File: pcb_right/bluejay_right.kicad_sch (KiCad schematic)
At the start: 60 parts, among them J2 SJ-43514, U2 MCP23017

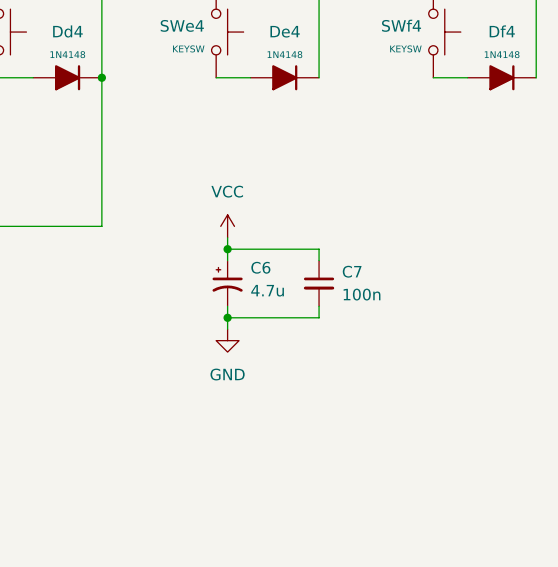
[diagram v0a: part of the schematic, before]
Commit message: Routing of right PCB
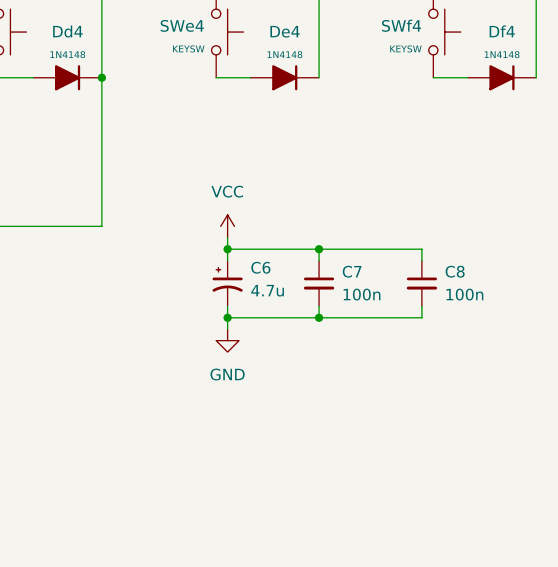
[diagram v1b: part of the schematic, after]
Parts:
- added C8: 100n, BlueJay footprints:C_Disc_D4.3mm_W1.9mm_P5.00mm, symbol BlueJaySymbolLibrary:C_Small
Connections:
- net GND: now also C8.2
- net VCC: now also C8.1
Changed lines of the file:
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@@
   (junction (at 146.05 62.23) (diameter 0) (color 0 0 0 0)
   )
+  (junction (at 229.87 111.76) (diameter 0) (color 0 0 0 0)
+  )
   (junction (at 219.71 111.76) (diameter 0) (color 0 0 0 0)
   )
@@
   )
   (junction (at 205.74 72.39) (diameter 0) (color 0 0 0 0)
+  )
+  (junction (at 229.87 104.14) (diameter 0) (color 0 0 0 0)
   )
   (junction (at 152.4 101.6) (diameter 0) (color 0 0 0 0)
@@
     (stroke (width 0) (type default) (color 0 0 0 0))
   )
+  (wire (pts (xy 241.3 111.76) (xy 241.3 110.49))
+    (stroke (width 0) (type default) (color 0 0 0 0))
+  )
   (wire (pts (xy 152.4 90.17) (xy 152.4 101.6))
     (stroke (width 0) (type default) (color 0 0 0 0))
@@
     (stroke (width 0) (type default) (color 0 0 0 0))
   )
+  (wire (pts (xy 229.87 111.76) (xy 241.3 111.76))
+    (stroke (width 0) (type default) (color 0 0 0 0))
+  )
   (wire (pts (xy 21.59 91.44) (xy 27.94 91.44))
     (stroke (width 0) (type default) (color 0 0 0 0))
@@
     (stroke (width 0) (type default) (color 0 0 0 0))
   )
+  (wire (pts (xy 229.87 104.14) (xy 241.3 104.14))
+    (stroke (width 0) (type default) (color 0 0 0 0))
+  )
   (wire (pts (xy 222.25 72.39) (xy 218.44 72.39))
     (stroke (width 0) (type default) (color 0 0 0 0))
@@
   )
   (wire (pts (xy 92.71 91.44) (xy 85.09 91.44))
+    (stroke (width 0) (type default) (color 0 0 0 0))
+  )
+  (wire (pts (xy 241.3 104.14) (xy 241.3 105.41))
     (stroke (width 0) (type default) (color 0 0 0 0))
   )
@@
     (pin "1")
   )
+  (symbol (lib_id "BlueJaySymbolLibrary:C_Small") (at 241.3 107.95 0) (unit 1)
+    (in_bom yes) (on_board yes) (fields_autoplaced)
+    (property "Reference" "C8" (id 0) (at 243.84 106.6862 0)
+      (effects (font (size 1.27 1.27)) (justify left))
+    )
+    (property "Value" "100n" (id 1) (at 243.84 109.2262 0)
+      (effects (font (size 1.27 1.27)) (justify left))
+    )
+    (property "Footprint" "BlueJay footprints:C_Disc_D4.3mm_W1.9mm_P5.00mm" (id 2) (at 241.3 107.95 0)
+      (effects (font (size 1.27 1.27)) hide)
+    )
+    (property "Datasheet" "~" (id 3) (at 241.3 107.95 0)
+      (effects (font (size 1.27 1.27)) hide)
+    )
+    (pin "1")
+    (pin "2")
+  )
   (symbol (lib_id "BlueJaySymbolLibrary:SJ-43514") (at 27.94 57.15 0) (unit 1)
     (in_bom yes) (on_board yes) (fields_autoplaced)
@@
       (reference "C7") (unit 1) (value "100n") (footprint "BlueJay footprints:C_Disc_D4.3mm_W1.9mm_P5.00mm")
     )
+    (path "/35a06a59-2769-4db8-80c5-5a4ade0be82e"
+      (reference "C8") (unit 1) (value "100n") (footprint "BlueJay footprints:C_Disc_D4.3mm_W1.9mm_P5.00mm")
+    )
     (path "/0a3ae171-fddc-48df-9a24-cb858ce40ad5"

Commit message: No need for decoupling cap on reset pin
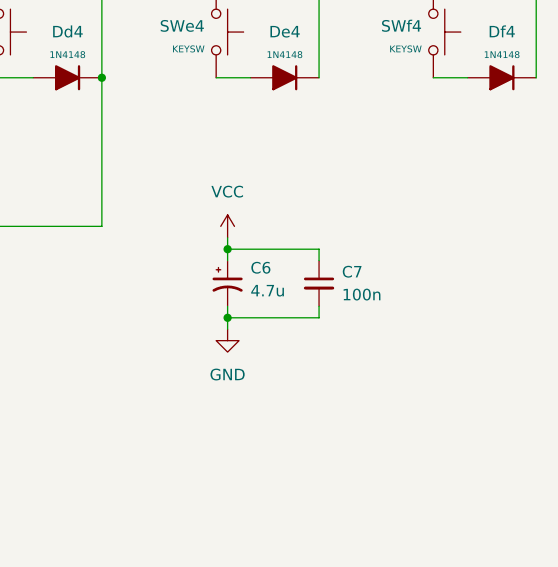
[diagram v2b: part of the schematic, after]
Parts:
- removed C8: 100n, BlueJay footprints:C_Disc_D4.3mm_W1.9mm_P5.00mm, symbol BlueJaySymbolLibrary:C_Small
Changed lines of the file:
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@@
   (junction (at 146.05 62.23) (diameter 0) (color 0 0 0 0)
   )
-  (junction (at 229.87 111.76) (diameter 0) (color 0 0 0 0)
-  )
   (junction (at 219.71 111.76) (diameter 0) (color 0 0 0 0)
   )
@@
   )
   (junction (at 205.74 72.39) (diameter 0) (color 0 0 0 0)
-  )
-  (junction (at 229.87 104.14) (diameter 0) (color 0 0 0 0)
   )
   (junction (at 152.4 101.6) (diameter 0) (color 0 0 0 0)
@@
     (stroke (width 0) (type default) (color 0 0 0 0))
   )
-  (wire (pts (xy 241.3 111.76) (xy 241.3 110.49))
-    (stroke (width 0) (type default) (color 0 0 0 0))
-  )
   (wire (pts (xy 152.4 90.17) (xy 152.4 101.6))
     (stroke (width 0) (type default) (color 0 0 0 0))
@@
     (stroke (width 0) (type default) (color 0 0 0 0))
   )
-  (wire (pts (xy 229.87 111.76) (xy 241.3 111.76))
-    (stroke (width 0) (type default) (color 0 0 0 0))
-  )
   (wire (pts (xy 21.59 91.44) (xy 27.94 91.44))
     (stroke (width 0) (type default) (color 0 0 0 0))
@@
     (stroke (width 0) (type default) (color 0 0 0 0))
   )
-  (wire (pts (xy 229.87 104.14) (xy 241.3 104.14))
-    (stroke (width 0) (type default) (color 0 0 0 0))
-  )
   (wire (pts (xy 222.25 72.39) (xy 218.44 72.39))
     (stroke (width 0) (type default) (color 0 0 0 0))
@@
   )
   (wire (pts (xy 92.71 91.44) (xy 85.09 91.44))
-    (stroke (width 0) (type default) (color 0 0 0 0))
-  )
-  (wire (pts (xy 241.3 104.14) (xy 241.3 105.41))
     (stroke (width 0) (type default) (color 0 0 0 0))
   )
@@
     (pin "1")
   )
-  (symbol (lib_id "BlueJaySymbolLibrary:C_Small") (at 241.3 107.95 0) (unit 1)
-    (in_bom yes) (on_board yes) (fields_autoplaced)
-    (property "Reference" "C8" (id 0) (at 243.84 106.6862 0)
-      (effects (font (size 1.27 1.27)) (justify left))
-    )
-    (property "Value" "100n" (id 1) (at 243.84 109.2262 0)
-      (effects (font (size 1.27 1.27)) (justify left))
-    )
-    (property "Footprint" "BlueJay footprints:C_Disc_D4.3mm_W1.9mm_P5.00mm" (id 2) (at 241.3 107.95 0)
-      (effects (font (size 1.27 1.27)) hide)
-    )
-    (property "Datasheet" "~" (id 3) (at 241.3 107.95 0)
-      (effects (font (size 1.27 1.27)) hide)
-    )
-    (pin "1")
-    (pin "2")
-  )
   (symbol (lib_id "BlueJaySymbolLibrary:SJ-43514") (at 27.94 57.15 0) (unit 1)
     (in_bom yes) (on_board yes) (fields_autoplaced)
@@
       (reference "C7") (unit 1) (value "100n") (footprint "BlueJay footprints:C_Disc_D4.3mm_W1.9mm_P5.00mm")
     )
-    (path "/35a06a59-2769-4db8-80c5-5a4ade0be82e"
-      (reference "C8") (unit 1) (value "100n") (footprint "BlueJay footprints:C_Disc_D4.3mm_W1.9mm_P5.00mm")
-    )
     (path "/0a3ae171-fddc-48df-9a24-cb858ce40ad5"
